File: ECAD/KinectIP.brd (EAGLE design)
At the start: 64.8 x 55.9 mm, 4 parts, among them P5+ 2PIN-FEMALE-HEADER

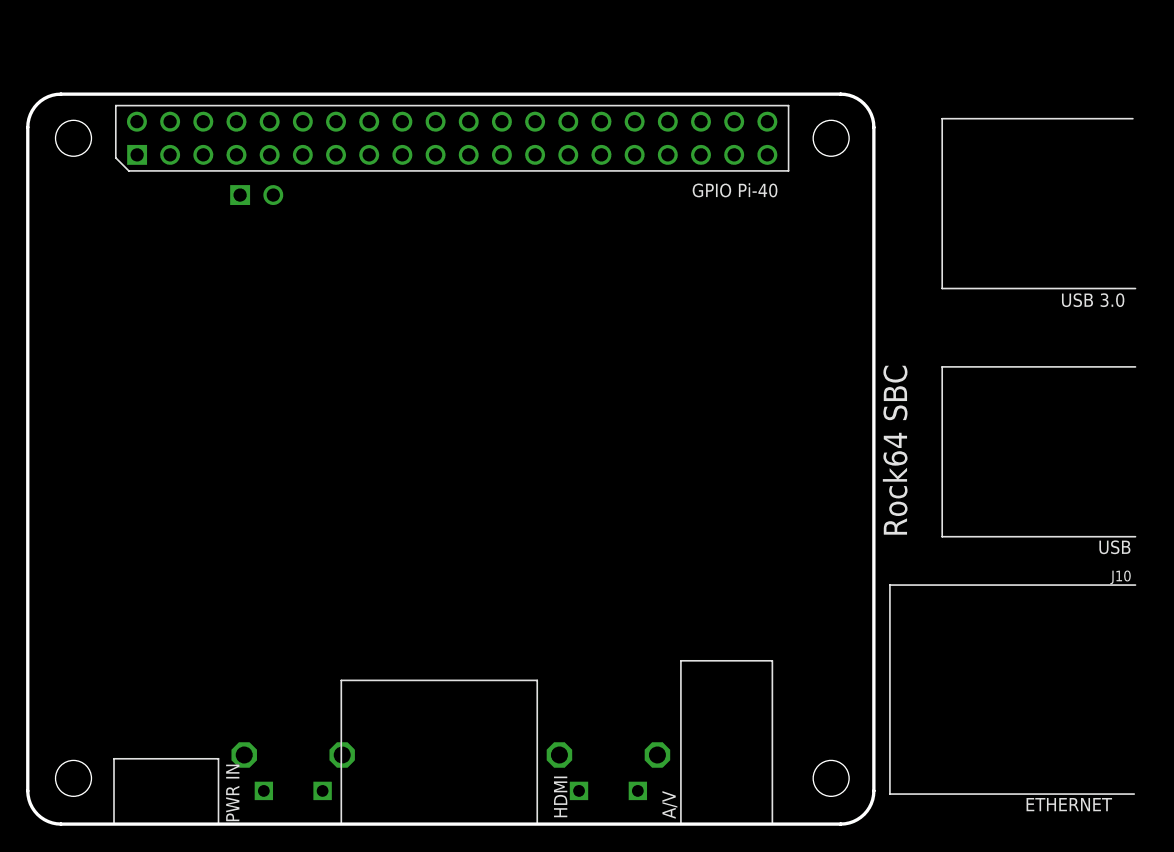
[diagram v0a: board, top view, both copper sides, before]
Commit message: add lbr
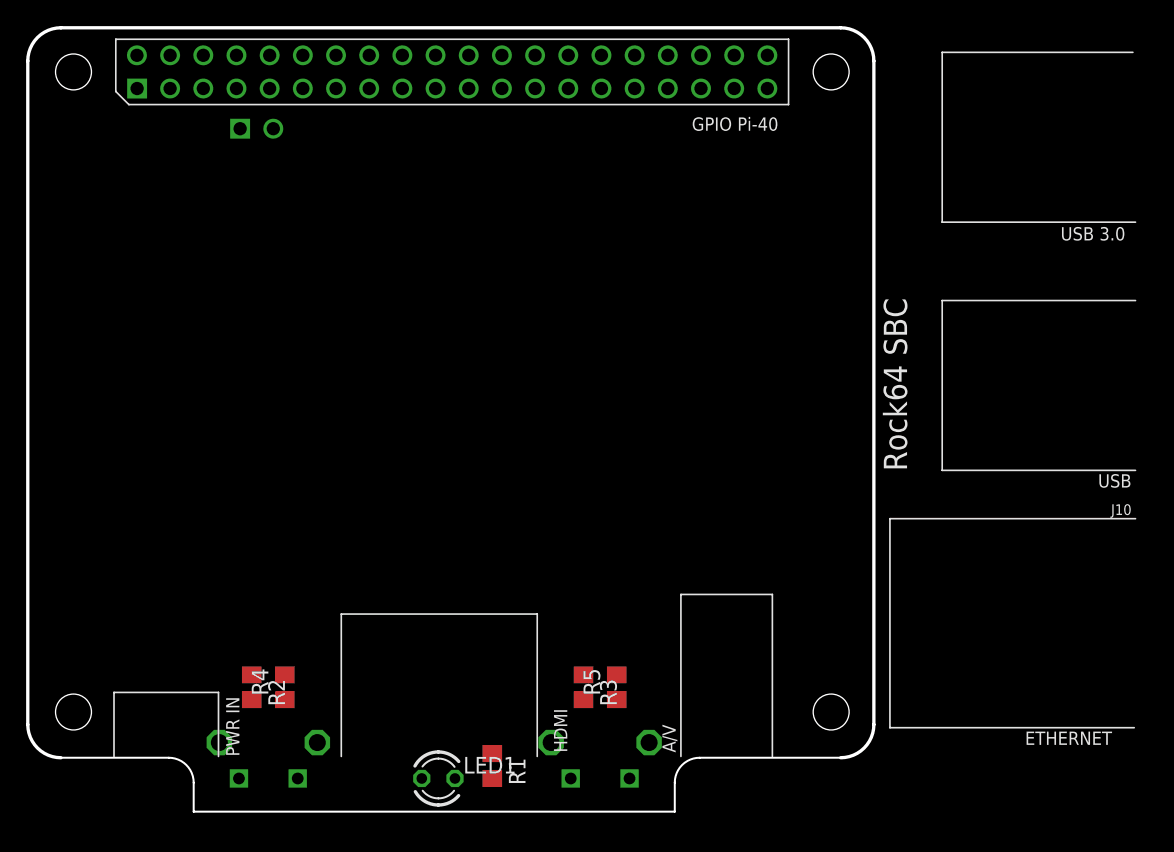
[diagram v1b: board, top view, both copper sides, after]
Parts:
- added LED1: (no value), led:LED3MM
- added R1, R4, R5: 330R, rcl:R0805
- added R2, R3: 10K, rcl:R0805
- moved PCB2 5.08 mm to (0.00, 5.08)
- moved P5+ 5.08 mm to (16.3, 53.2)
- moved ID 2.13 mm to (18.4, 3.49)
- moved PWR 1.14 mm to (43.8, 3.49)
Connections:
- new net +3V3: PCB2.P$1, R4.2, R5.2
- new net 0V: ID.MNT$1, ID.MNT$2, PCB2.P$25, PWR.MNT$1, PWR.MNT$2, R1.1, R2.1, R3.1
- new net N$1: LED1.A, PCB2.P$15
- new net N$2: LED1.K, R1.2
- new net N$3: ID.SW$2, R4.1
- new net N$4: PWR.SW$2, R5.1
- new net N$5: ID.SW$1, P5+.P$1, R2.2
- new net N$6: P5+.P$2, PWR.SW$1, R3.2
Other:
- board size 64.8 x 55.9 mm -> 64.8 x 60 mm
